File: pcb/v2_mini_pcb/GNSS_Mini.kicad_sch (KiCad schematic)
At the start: 16 parts, among them J1 Conn_Coaxial, U1 UM980

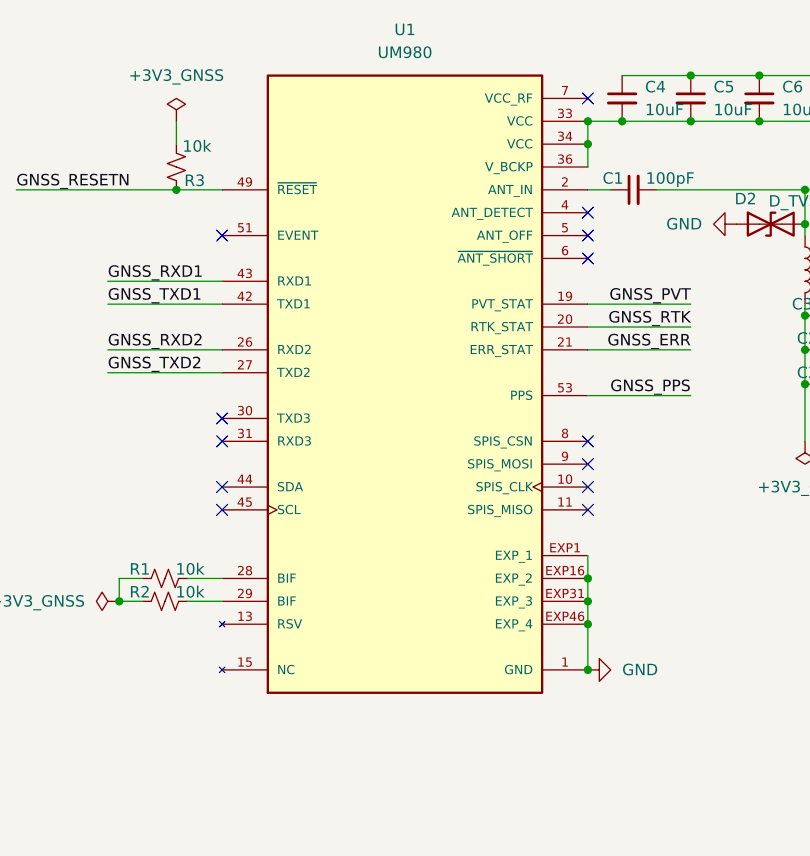
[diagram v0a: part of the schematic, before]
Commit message: fix minor edc rules
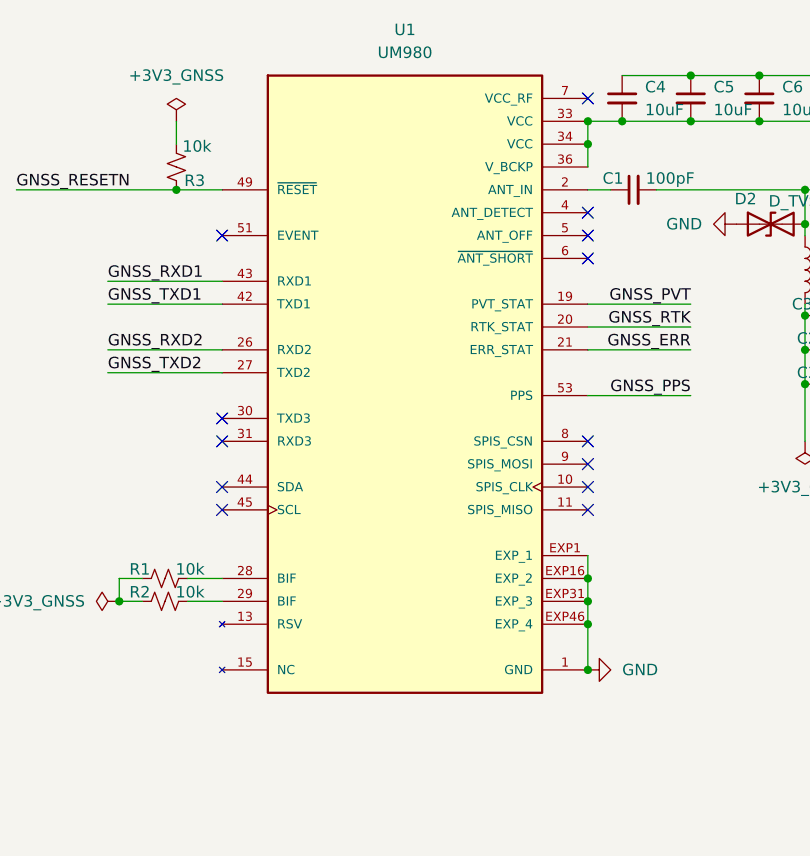
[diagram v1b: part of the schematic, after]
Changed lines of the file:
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@@
 		(pin "34"
-		)
-		(pin "29"
 		)
 		(instances
@@
 	)
 	(symbol
+		(lib_id "Device:R_Small_US")
+		(at 59.69 113.03 90)
+		(unit 1)
+		(body_style 1)
+		(exclude_from_sim no)
+		(in_bom yes)
+		(on_board yes)
+		(in_pos_files yes)
+		(dnp no)
+		(property "Reference" "R2"
+			(at 56.896 112.014 90)
+			(show_name no)
+			(do_not_autoplace no)
+			(effects
+				(font
+					(size 1.27 1.27)
+				)
+			)
+		)
+		(property "Value" "10k"
+			(at 62.484 112.014 90)
+			(show_name no)
+			(do_not_autoplace no)
+			(effects
+				(font
+					(size 1.27 1.27)
+				)
+			)
+		)
+		(property "Footprint" ""
+			(at 59.69 113.03 0)
+			(hide yes)
+			(show_name no)
+			(do_not_autoplace no)
+			(effects
+				(font
+					(size 1.27 1.27)
+				)
+			)
+		)
+		(property "Datasheet" ""
+			(at 59.69 113.03 0)
+			(hide yes)
+			(show_name no)
+			(do_not_autoplace no)
+			(effects
+				(font
+					(size 1.27 1.27)
+				)
+			)
+		)
+		(property "Description" "Resistor, small US symbol"
+			(at 59.69 113.03 0)
+			(hide yes)
+			(show_name no)
+			(do_not_autoplace no)
+			(effects
+				(font
+					(size 1.27 1.27)
+				)
+			)
+		)
+		(pin "2"
+		)
+		(pin "1"
+		)
+		(instances
+			(project "v2_mini"
+				(path "/4318b369-034c-40ef-a05b-b7d2541c0647/a81c2312-17da-4077-8f80-7b7fd8fe19c5"
+					(reference "R2")
+					(unit 1)
+				)
+			)
+		)
+	)
+	(symbol
 		(lib_id "power:GND")
 		(at 143.51 72.39 0)
@@
 					(unit 1)
 				)
-			)
-		)
-	)
-	(symbol
-		(lib_id "Device:R_Small_US")
-		(at 59.69 113.03 90)
-		(unit 1)
-		(body_style 1)
-		(exclude_from_sim no)
-		(in_bom yes)
-		(on_board yes)
-		(in_pos_files yes)
-		(dnp no)
-		(property "Reference" "R2"
-			(at 56.896 112.014 90)
-			(show_name no)
-			(do_not_autoplace no)
-			(effects
-				(font
-					(size 1.27 1.27)
-				)
-			)
-		)
-		(property "Value" "10k"
-			(at 62.484 112.014 90)
-			(show_name no)
-			(do_not_autoplace no)
-			(effects
-				(font
-					(size 1.27 1.27)
-				)
-			)
-		)
-		(property "Footprint" ""
-			(at 59.69 113.03 0)
-			(hide yes)
-			(show_name no)
-			(do_not_autoplace no)
-			(effects
-				(font
-					(size 1.27 1.27)
-				)
-			)
-		)
-		(property "Datasheet" ""
-			(at 59.69 113.03 0)
-			(hide yes)
-			(show_name no)
-			(do_not_autoplace no)
-			(effects
-				(font
-					(size 1.27 1.27)
-				)
-			)
-		)
-		(property "Description" "Resistor, small US symbol"
-			(at 59.69 113.03 0)
-			(hide yes)
-			(show_name no)
-			(do_not_autoplace no)
-			(effects
-				(font
-					(size 1.27 1.27)
-				)
-			)
-		)
-		(pin "2"
-		)
-		(pin "1"
-		)
-		(instances
-			(project "v2_mini"
-				(path "/4318b369-034c-40ef-a05b-b7d2541c0647/a81c2312-17da-4077-8f80-7b7fd8fe19c5"
-					(reference "R2")
-					(unit 1)
-				)

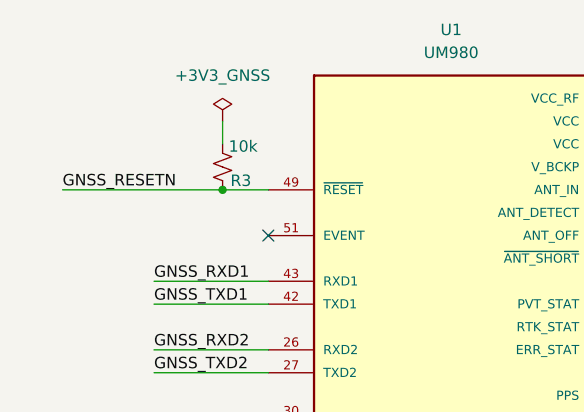
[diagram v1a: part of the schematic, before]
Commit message: erc rules
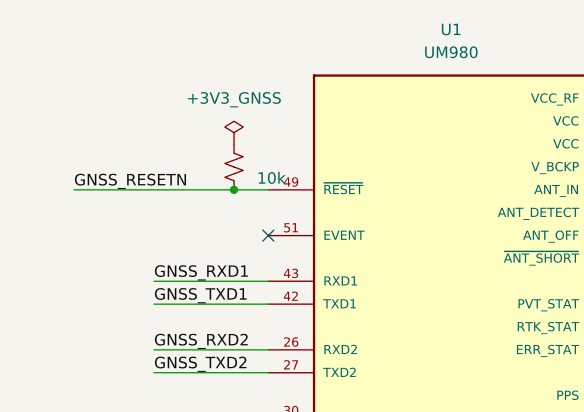
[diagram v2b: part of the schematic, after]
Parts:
- removed R3: 10k, symbol Device:R_Small_US
- added R24: 10k, symbol Device:R_Small_US
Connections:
- net GNSS_RESETN: now also R24.1

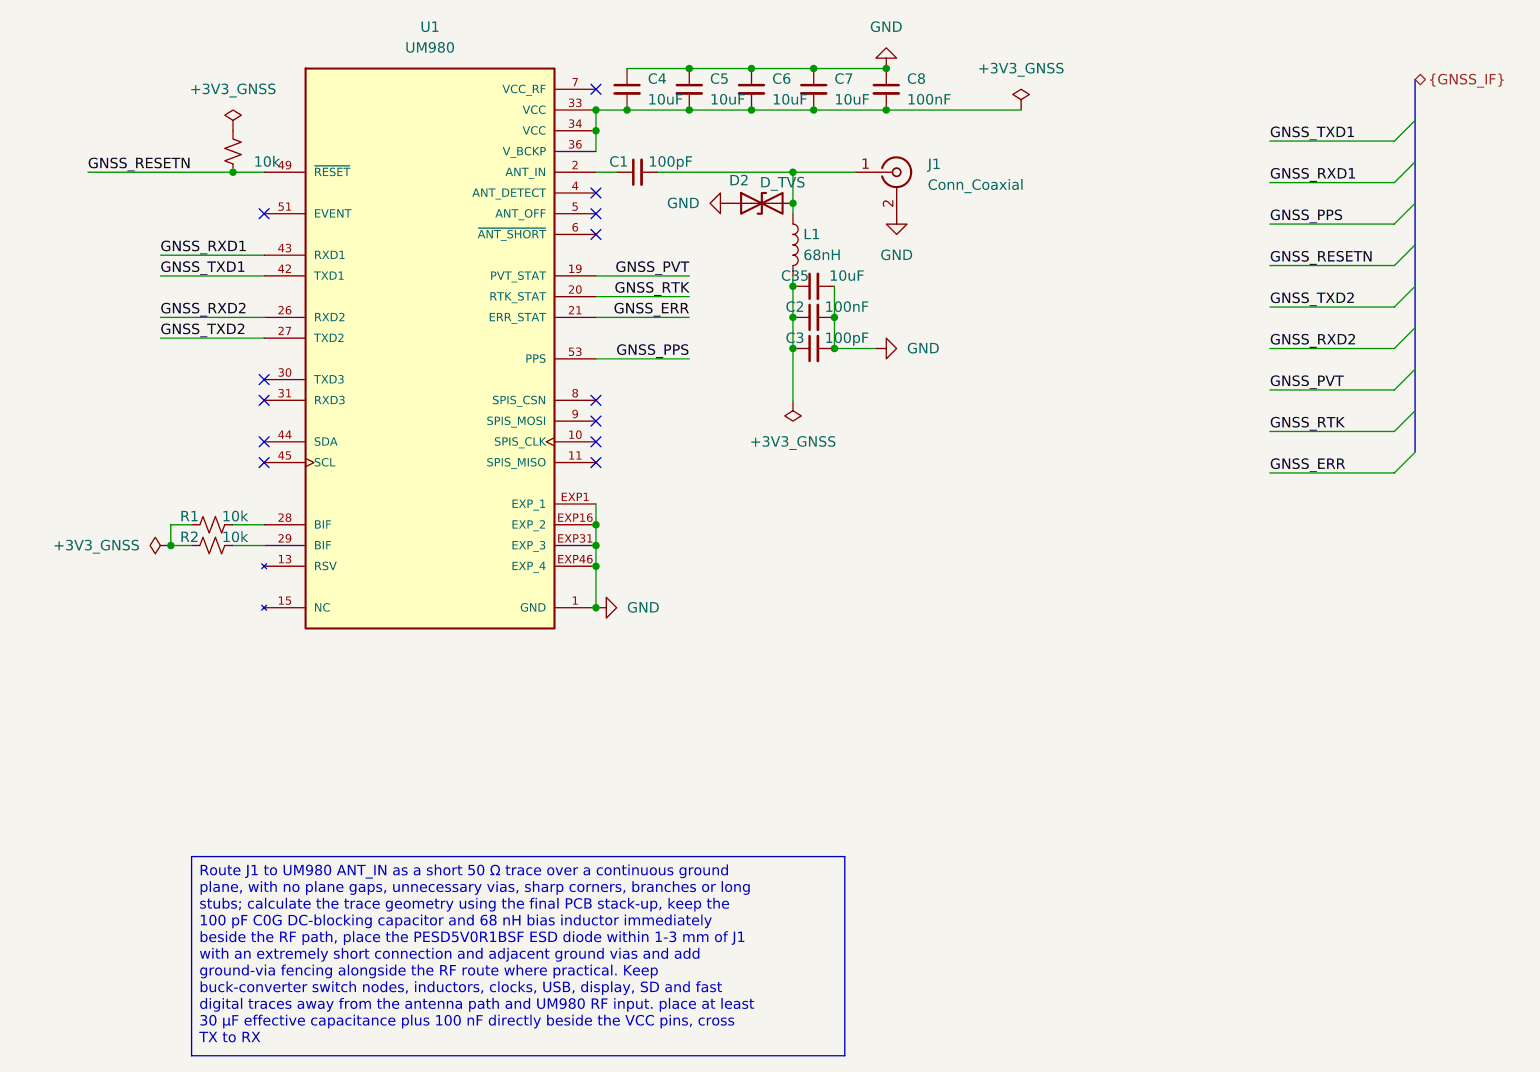
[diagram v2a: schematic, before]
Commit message: update pcb issues
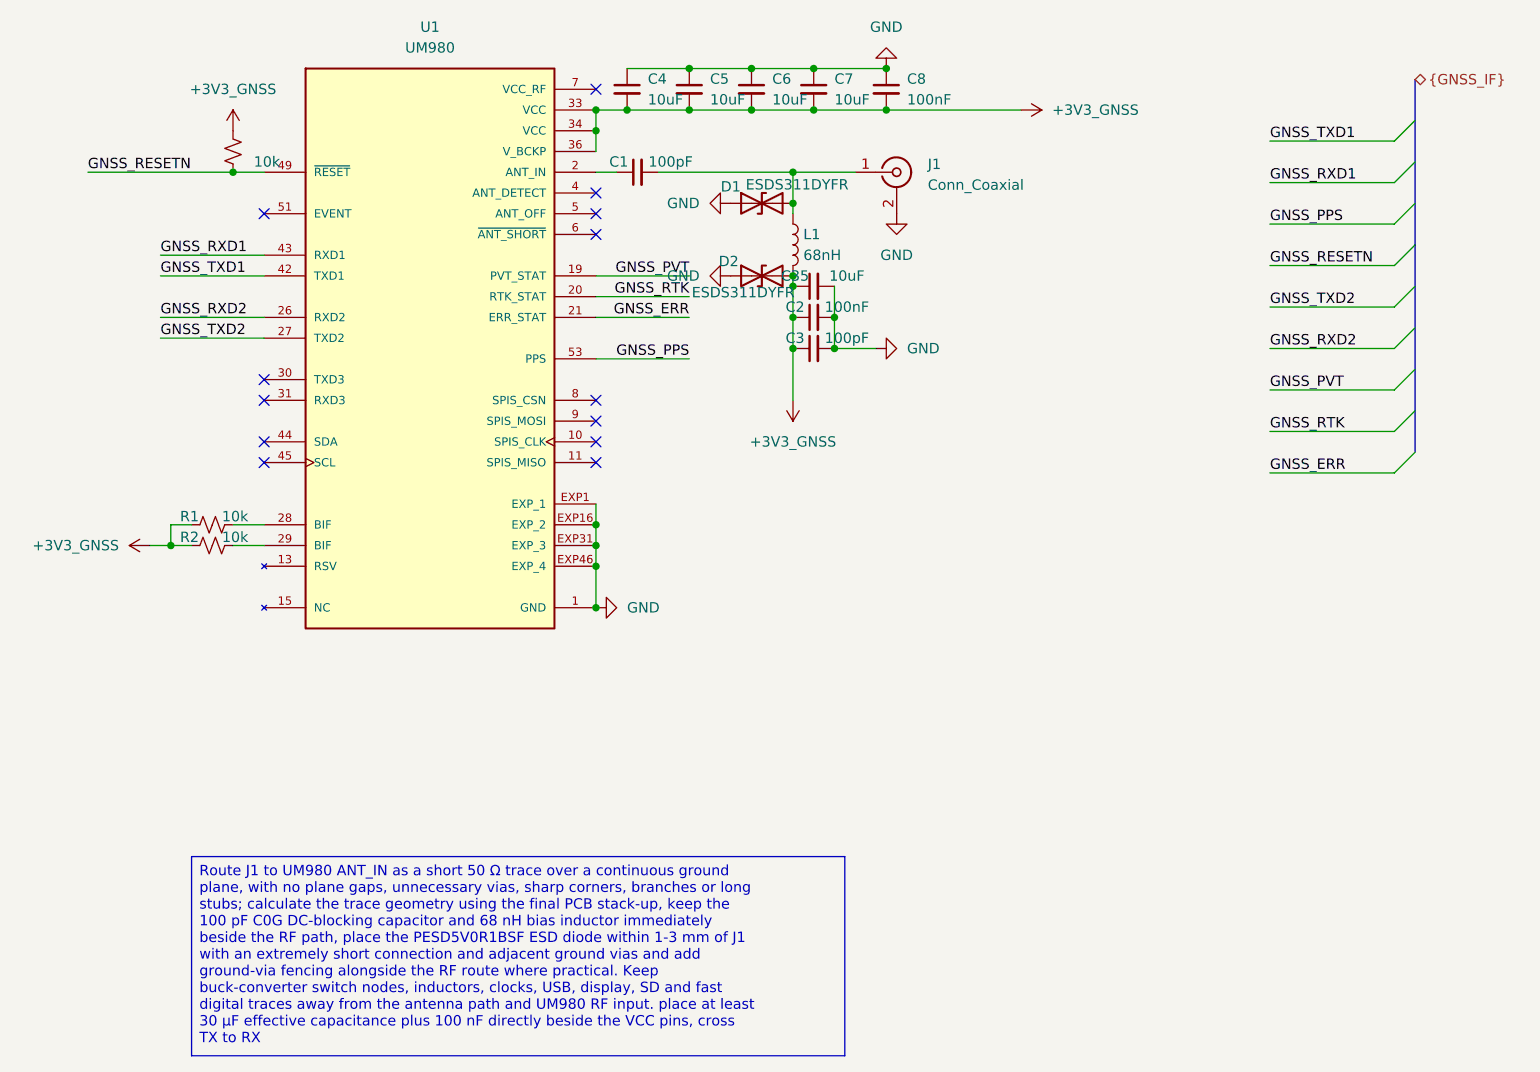
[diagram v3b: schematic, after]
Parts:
- added D1: ESDS311DYFR, symbol Device:D_TVS
- D2: value D_TVS -> ESDS311DYFR
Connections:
- net VCC is gone; now on net +3V3_GNSS: C4.2, C5.2, C6.2, C7.2, C8.2, U1.33 (VCC), U1.34 (VCC), U1.36 (V_BCKP)
- net EXP_1: now also D1.1 (A1)
- net +3V3_GNSS: now reaches C2.1, C3.1, C35.1, L1.2
- net +3V3_GNSS: now also D2.2 (A2), R1.1, R2.1, R24.2
- net at C1.2, J1.1 (In), L1.1: now also D1.2 (A2); no longer D2.2 (A2)

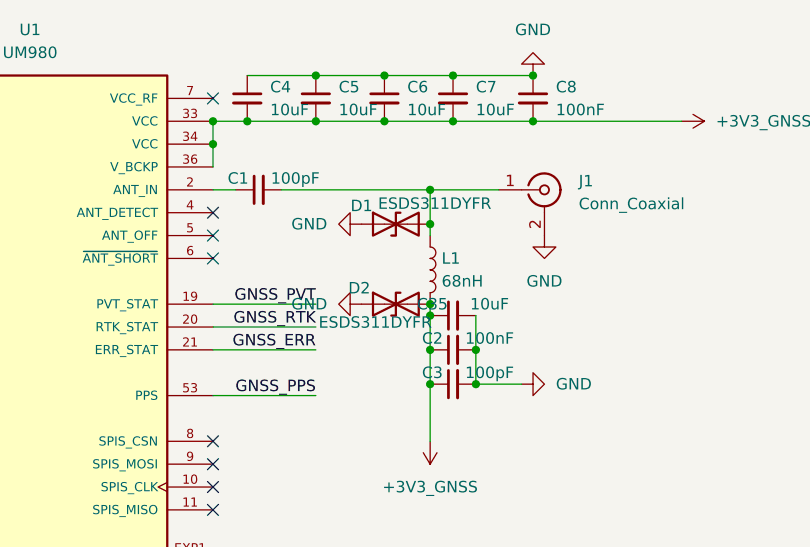
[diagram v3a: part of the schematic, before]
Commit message: add mpn and footprints for some
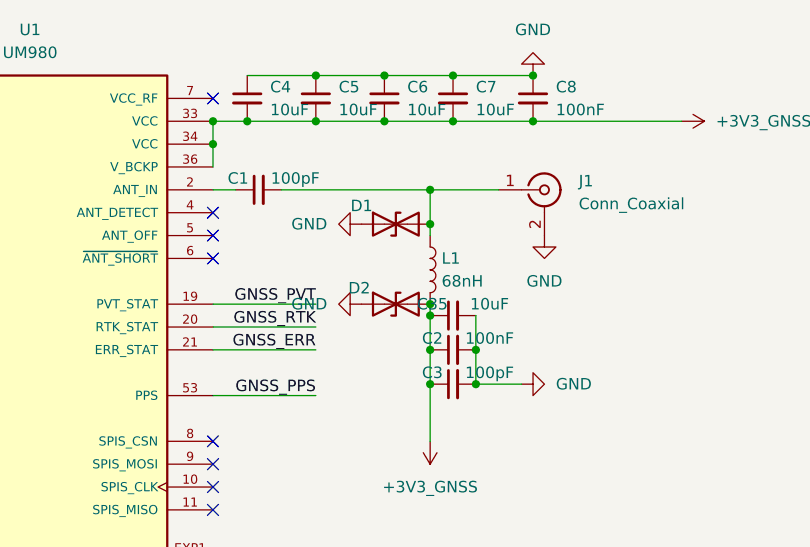
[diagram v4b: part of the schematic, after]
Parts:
- C1, C3: footprint (none) -> Capacitor_SMD:C_01005_0402Metric; MPN (none) -> 0402CG101J500NT
- C2, C8: footprint (none) -> Capacitor_SMD:C_01005_0402Metric; MPN (none) -> CL05B104KB54PNC
- C35, C4, C5, C6, C7: footprint (none) -> Capacitor_SMD:C_0201_0603Metric; MPN (none) -> CL10A106KP8NNNC
- D1: value ESDS311DYFR -> (none); footprint (none) -> Package_SON:Texas_DPY0002A_0.6x1mm_P0.65mm; MPN (none) -> TPD1E0B04DPYR
- D2: value ESDS311DYFR -> (none); footprint (none) -> Diode_SMD:D_SOD-323F; MPN (none) -> ESDS311DYFR
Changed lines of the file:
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@@
 			)
 		)
-		(property "Footprint" ""
+		(property "Footprint" "Capacitor_SMD:C_01005_0402Metric"
 			(at 142.24 57.15 0)
 			(hide yes)
@@
 		)
 		(property "Description" "Unpolarized capacitor, small symbol"
+			(at 142.24 57.15 0)
+			(hide yes)
+			(show_name no)
+			(do_not_autoplace no)
+			(effects
+				(font
+					(size 1.27 1.27)
+				)
+			)
+		)
+		(property "MPN" "CL05B104KB54PNC"
 			(at 142.24 57.15 0)
 			(hide yes)
@@
 			)
 		)
-		(property "Footprint" ""
+		(property "Footprint" "Capacitor_SMD:C_0201_0603Metric"
 			(at 118.11 57.15 0)
 			(hide yes)
@@
 		)
 		(property "Description" "Unpolarized capacitor, small symbol"
+			(at 118.11 57.15 0)
+			(hide yes)
+			(show_name no)
+			(do_not_autoplace no)
+			(effects
+				(font
+					(size 1.27 1.27)
+				)
+			)
+		)
+		(property "MPN" "CL10A106KP8NNNC"
 			(at 118.11 57.15 0)
 			(hide yes)
@@
 			)
 		)
-		(property "Footprint" ""
+		(property "Footprint" "Capacitor_SMD:C_0201_0603Metric"
 			(at 133.35 81.28 0)
 			(hide yes)
@@
 		(property "Description" "Unpolarized capacitor, small symbol"
 			(at 133.35 81.28 0)
+			(hide yes)
+			(show_name no)
+			(do_not_autoplace no)
+			(effects
+				(font
+					(size 1.27 1.27)
+				)
+			)
+		)
+		(property "MPN" "CL10A106KP8NNNC"
+			(at 133.35 81.28 90)
 			(hide yes)
 			(show_name no)
@@
 			)
 		)
-		(property "Value" "ESDS311DYFR"
+		(property "Value" ""
 			(at 124.714 82.042 0)
 			(show_name no)
@@
 			)
 		)
-		(property "Footprint" ""
+		(property "Footprint" "Diode_SMD:D_SOD-323F"
 			(at 127 80.01 0)
 			(hide yes)
@@
 		)
 		(property "Description" "Bidirectional transient-voltage-suppression diode"
+			(at 127 80.01 0)
+			(hide yes)
+			(show_name no)
+			(do_not_autoplace no)
+			(effects
+				(font
+					(size 1.27 1.27)
+				)
+			)
+		)
+		(property "MPN" "ESDS311DYFR"
 			(at 127 80.01 0)
 			(hide yes)
@@
 			)
 		)
+		(property "MPN" ""
+			(at 59.69 110.49 90)
+			(hide yes)
+			(show_name no)
+			(do_not_autoplace no)
+			(effects
+				(font
+					(size 1.27 1.27)
+				)
+			)
+		)
 		(pin "2"
 		)
@@
 			)
 		)
-		(property "Footprint" ""
+		(property "Footprint" "Capacitor_SMD:C_01005_0402Metric"
 			(at 111.76 67.31 0)
 			(hide yes)
@@
 		(property "Description" "Unpolarized capacitor, small symbol"
 			(at 111.76 67.31 0)
+			(hide yes)
+			(show_name no)
+			(do_not_autoplace no)
+			(effects
+				(font
+					(size 1.27 1.27)
+				)
+			)
+		)
+		(property "MPN" "0402CG101J500NT"
+			(at 111.76 67.31 90)
 			(hide yes)
 			(show_name no)
@@
 			)
 		)
+		(property "MPN" ""
+			(at 62.23 64.77 0)
+			(hide yes)
+			(show_name no)
+			(do_not_autoplace no)
+			(effects
+				(font
+					(size 1.27 1.27)
+				)
+			)
+		)
 		(pin "1"
 		)
@@
 			)
 		)
+		(property "MPN" ""
+			(at 86.36 87.63 0)
+			(hide yes)
+			(show_name no)
+			(do_not_autoplace no)
+			(effects
+				(font
+					(size 1.27 1.27)
+				)
+			)
+		)
 		(pin "11"
 		)
@@
 			)
 		)
+		(property "MPN" ""
+			(at 143.51 67.31 0)
+			(hide yes)
+			(show_name no)
+			(do_not_autoplace no)
+			(effects
+				(font
+					(size 1.27 1.27)
+				)
+			)
+		)
 		(pin "1"
 		)
@@
 		(property "Description" "Resistor, small US symbol"
 			(at 59.69 113.03 0)
+			(hide yes)
+			(show_name no)
+			(do_not_autoplace no)
+			(effects
+				(font
+					(size 1.27 1.27)
+				)
+			)
+		)
+		(property "MPN" ""
+			(at 59.69 113.03 90)
 			(hide yes)
 			(show_name no)
@@
 			)
 		)
-		(property "Value" "ESDS311DYFR"
+		(property "Value" ""
 			(at 131.318 68.834 0)
 			(show_name no)
@@
 			)
 		)
-		(property "Footprint" ""
+		(property "Footprint" "Package_SON:Texas_DPY0002A_0.6x1mm_P0.65mm"
 			(at 127 71.12 0)
 			(hide yes)
@@
 		)
 		(property "Description" "Bidirectional transient-voltage-suppression diode"
+			(at 127 71.12 0)
+			(hide yes)
+			(show_name no)
+			(do_not_autoplace no)
+			(effects
+				(font
+					(size 1.27 1.27)
+				)
+			)
+		)
+		(property "MPN" "TPD1E0B04DPYR"
 			(at 127 71.12 0)
 			(hide yes)
@@
 			)
 		)
-		(property "Footprint" ""
+		(property "Footprint" "Capacitor_SMD:C_01005_0402Metric"
 			(at 133.35 85.09 0)
 			(hide yes)
@@
 		(property "Description" "Unpolarized capacitor, small symbol"
 			(at 133.35 85.09 0)
+			(hide yes)
+			(show_name no)
+			(do_not_autoplace no)
+			(effects
+				(font
+					(size 1.27 1.27)
+				)
+			)
+		)
+		(property "MPN" "CL05B104KB54PNC"
+			(at 133.35 85.09 90)
 			(hide yes)
 			(show_name no)
@@
 			)
 		)
-		(property "Footprint" ""
+		(property "Footprint" "Capacitor_SMD:C_01005_0402Metric"
 			(at 133.35 88.9 0)
 			(hide yes)
@@
 		(property "Description" "Unpolarized capacitor, small symbol"
 			(at 133.35 88.9 0)
+			(hide yes)
+			(show_name no)
+			(do_not_autoplace no)
+			(effects
+				(font
+					(size 1.27 1.27)
+				)
+			)
+		)
+		(property "MPN" "0402CG101J500NT"
+			(at 133.35 88.9 90)
 			(hide yes)
 			(show_name no)
@@
 			)
 		)
-		(property "Footprint" ""
+		(property "Footprint" "Capacitor_SMD:C_0201_0603Metric"
 			(at 110.49 57.15 0)
 			(hide yes)
@@
 		)
 		(property "Description" "Unpolarized capacitor, small symbol"
+			(at 110.49 57.15 0)
+			(hide yes)
+			(show_name no)
+			(do_not_autoplace no)
+			(effects
+				(font
+					(size 1.27 1.27)
+				)
+			)
+		)
+		(property "MPN" "CL10A106KP8NNNC"
 			(at 110.49 57.15 0)
 			(hide yes)
@@
 			)
 		)
+		(property "MPN" ""
+			(at 130.81 76.2 0)
+			(hide yes)
+			(show_name no)
+			(do_not_autoplace no)
+			(effects
+				(font
+					(size 1.27 1.27)
+				)
+			)
+		)
 		(pin "1"
 		)
@@
 			)
 		)
-		(property "Footprint" ""
+		(property "Footprint" "Capacitor_SMD:C_0201_0603Metric"
 			(at 133.35 57.15 0)
 			(hide yes)
@@
 		)
 		(property "Description" "Unpolarized capacitor, small symbol"
+			(at 133.35 57.15 0)
+			(hide yes)
+			(show_name no)
+			(do_not_autoplace no)
+			(effects
+				(font
+					(size 1.27 1.27)
+				)
+			)
+		)
+		(property "MPN" "CL10A106KP8NNNC"
 			(at 133.35 57.15 0)
 			(hide yes)
@@
 			)
 		)
-		(property "Footprint" ""
+		(property "Footprint" "Capacitor_SMD:C_0201_0603Metric"
 			(at 125.73 57.15 0)
 			(hide yes)
@@
 			(at 125.73 57.15 0)
 			(hide yes)
+			(show_name no)
+			(do_not_autoplace no)
+			(effects
+				(font
+					(size 1.27 1.27)
+				)
+			)
+		)
+		(property "MPN" "CL10A106KP8NNNC"
+			(at 125.73 57.15 0)
+			(hide yes)
